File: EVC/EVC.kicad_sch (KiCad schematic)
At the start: 31 parts, among them CN1 HC-ZH1.5-6AW, CN2 HC-ZH1.5-6AW, CN3 HC-ZH1.5-6AW, CN4 HC-ZH1.5-6AW, J1 USB4105-GF-A, U1 CH592X, U2 TCR2EF33_LMCT, U3 C30732.768NCXE20, U4 DRV8835DSSR, U5 DRV8835DSSR, U6 ANT3216LL00R2400A, Y1 XRCGB32M000F2P01R0

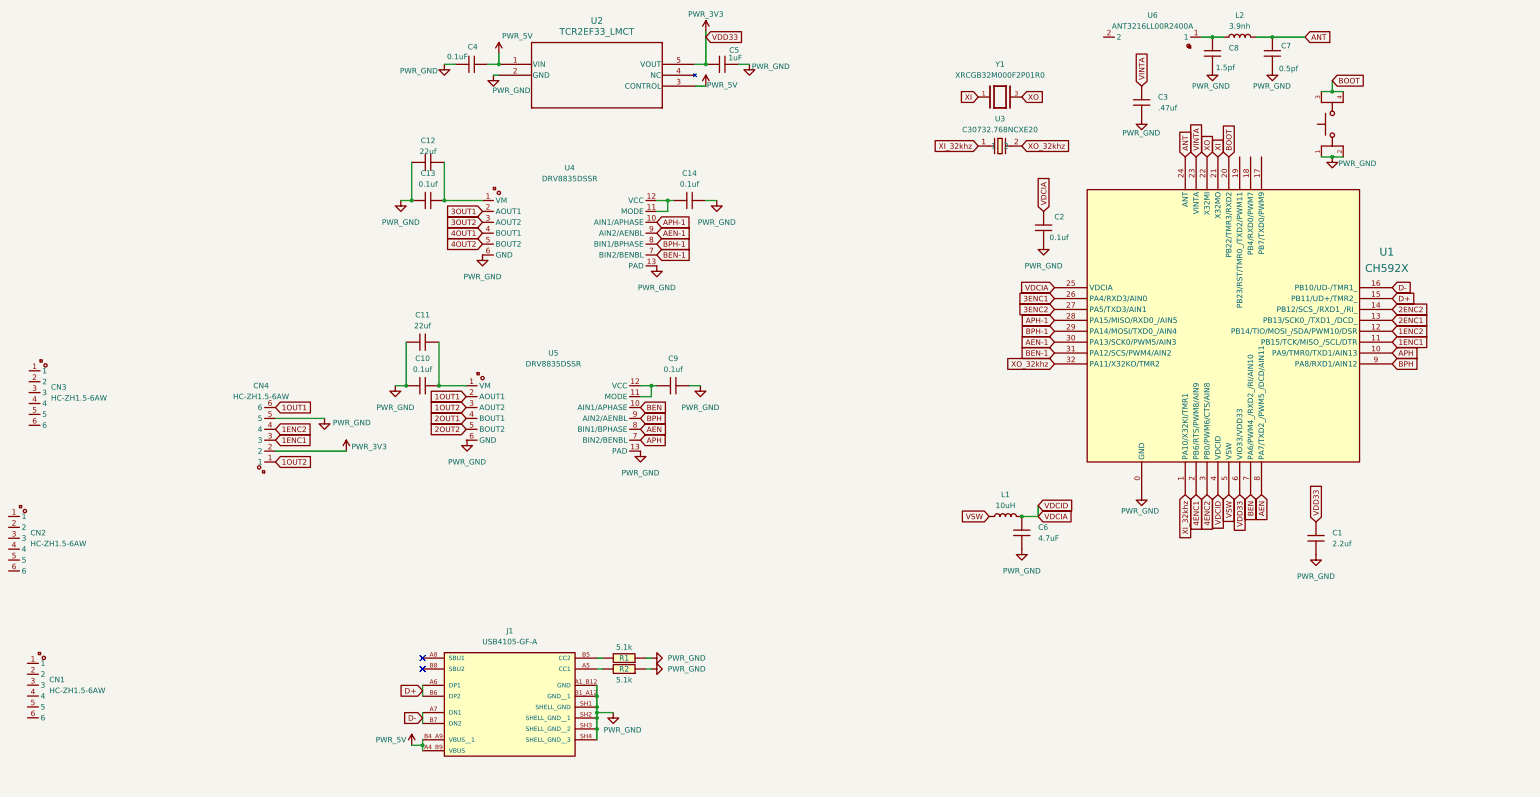
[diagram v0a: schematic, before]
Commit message: done
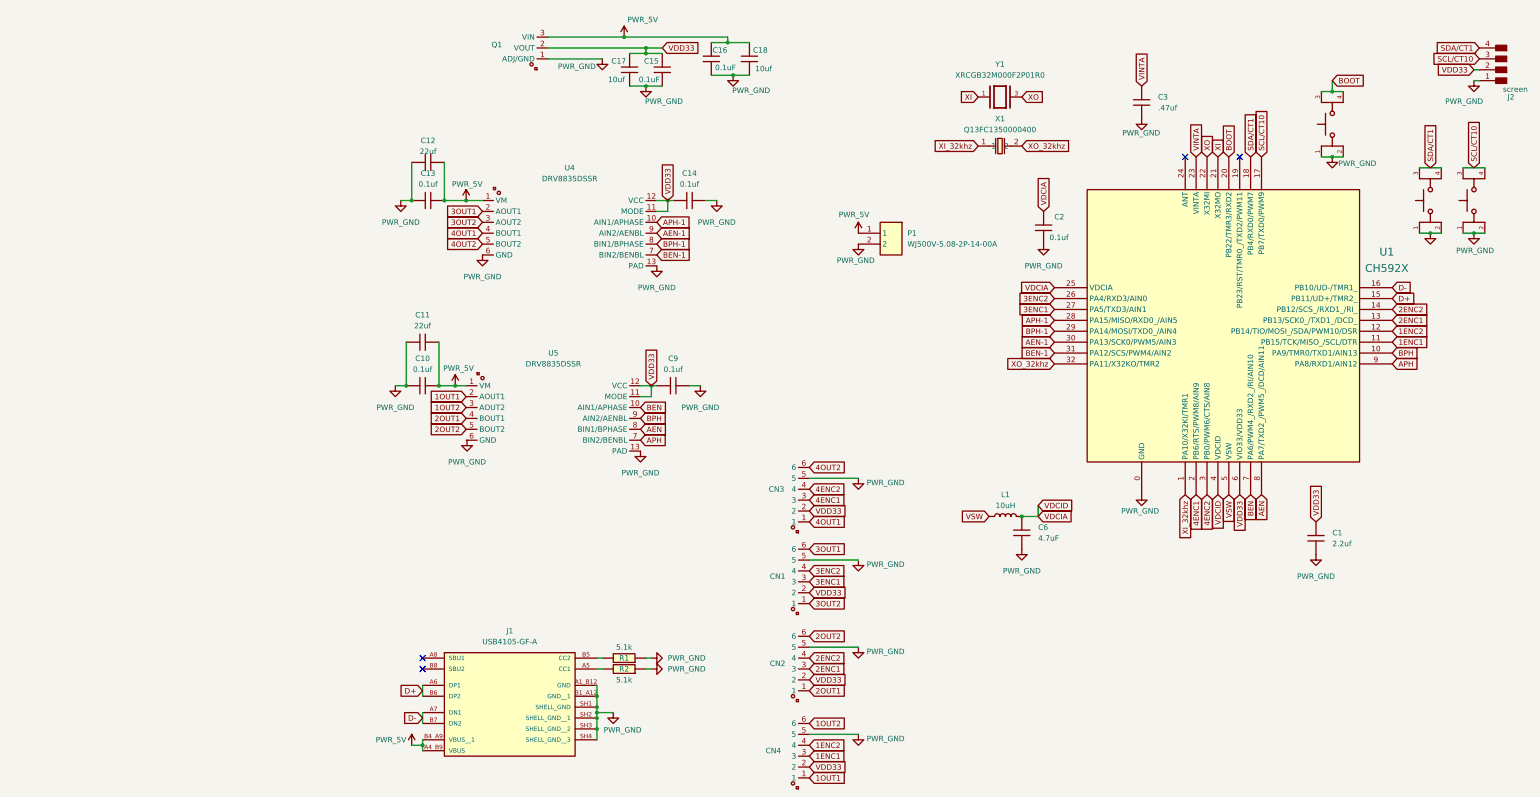
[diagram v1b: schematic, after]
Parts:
- removed C4: 0.1uF, Footprint:C_0603, symbol fab:C_0603
- removed C5: 1uF, Footprint:C_0603, symbol fab:C_0603
- removed C7: 0.5pf, Footprint:C_0603, symbol fab:C_0603
- removed C8: 1.5pf, Footprint:C_0603, symbol fab:C_0603
- removed L2: 3.9nh, Footprint:0603, symbol 0603:L_0603
- removed U2: TCR2EF33_LMCT, Footprint:voltage regulator, symbol voltage regulator:TCR2EF33_LMCT
- removed U3: C30732.768NCXE20, EasyEDA:HC-49S_L7.2-W3.2, symbol EasyEDA:C30732.768NCXE20
- removed U6: ANT3216LL00R2400A, EasyEDA:ANT-SMD_L3.2-W1.6, symbol EasyEDA:ANT3216LL00R2400A
- added C15, C16: 0.1uF, Footprint:C_0603, symbol fab:C_0603
- added C17, C18: 10uf, Footprint:C_0603, symbol fab:C_0603
- added J2: screen, Footprint:PinHeader_01x04_P2.54mm_Vertical_THT_D1mm, symbol fab:PinHeader_01x04_P2.54mm_Vertical_THT_D1mm
- added P1: WJ500V-5.08-2P-14-00A, EasyEDA:CONN-TH_2P-P5.00_WJ500V-5.08-2P, symbol EasyEDA:WJ500V-5.08-2P-14-00A
- added Q1: AMS1117-3.3V_C5120796, EasyEDA:SOT-89-3_L4.5-W2.5-P1.50-LS4.2-BR, symbol EasyEDA:AMS1117-3.3V_C5120796
- added S1, S3: TL3365AF180QG, Footprint:button, symbol button:TL3365AF180QG
- added X1: Q13FC1350000400, EasyEDA:FC-135R_L3.2-W1.5, symbol EasyEDA:Q13FC1350000400
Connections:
- net PWR_3V3 is gone; now on net VDD33: C1.1, CN4.2, U1.6 (VIO33/VDD33)
- net 1OUT1: now also CN4.1; no longer CN4.6
- net 1OUT2: now also CN4.6; no longer CN4.1
- net 2ENC1: now also CN2.3
- net 2ENC2: now also CN2.4
- net 2OUT1: now also CN2.1
- net 2OUT2: now also CN2.6
- net 3ENC1: now also CN1.3, U1.27 (PA5/TXD3/AIN1); no longer U1.26 (PA4/RXD3/AIN0)
- net 3ENC2: now also CN1.4, U1.26 (PA4/RXD3/AIN0); no longer U1.27 (PA5/TXD3/AIN1)
- net 3OUT1: now also CN1.6
- net 3OUT2: now also CN1.1
- net 4ENC1: now also CN3.3
- net 4ENC2: now also CN3.4
- net 4OUT1: now also CN3.1
- net 4OUT2: now also CN3.6
- net APH: now also U1.9 (PA8/RXD1/AIN12); no longer U1.10 (PA9/TMR0/TXD1/AIN13)
- net BPH: now also U1.10 (PA9/TMR0/TXD1/AIN13); no longer U1.9 (PA8/RXD1/AIN12)
- net PWR_5V: now also C10.2, C11.2, C12.2, C13.2, U4.1 (VM), U5.1 (VM), C16.2, C18.2, P1.1, Q1.3 (VIN)
- net PWR_GND: now also CN1.5, CN2.5, CN3.5, C15.1, C16.1, C17.1, C18.1, J2.1 (Pin_1), P1.2, Q1.1 (ADJ/GND), S1.1, S1.2, S3.1, S3.2
- net XI_32khz: now also X1.1
- net XO_32khz: now also X1.2
- net VDD33: now reaches C9.1, U5.11 (MODE), U5.12 (VCC)
- net VDD33: now also C14.1, CN1.2, CN2.2, CN3.2, U4.11 (MODE), U4.12 (VCC), C15.2, C17.2, J2.2 (Pin_2), Q1.2 (VOUT)
- net SCL/CT10: now reaches U1.17 (PB7/TXD0/PWM9)
- net SCL/CT10: now also J2.3 (Pin_3), S3.3, S3.4
- net SDA/CT1: now reaches U1.18 (PB4/RXD0/PWM7)
- net SDA/CT1: now also J2.4 (Pin_4), S1.3, S1.4
- net ANT: no longer names the net of U1.24 (ANT)
- no-connect marks 2 -> 4
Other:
- moved on the sheet: CN1, CN2, CN3, CN4
